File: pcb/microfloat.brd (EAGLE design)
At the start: 76.2 x 60.3 mm, 156 parts, among them J1 503182-1852, J2 1054291110, J3 USB4105_REVA, J4 1054291110, J5 JTAG-MINI, J6 1909763-1, J7 1054291110, J8 1054291110, T100 MMBT3906, U1 TXB0104PWR, U100 TPS54308DDCT, U101 LTC4419CMSEPBF, U102 MAX13237EETE, U103 TPS54308DDCT, U104 TPS54308DDCT, U105 TPS54308DDCT, U2 ICM-42688-P, U3 ATSAMD51N20A-AUT, U4 NEO-M8N-0, U5 BME280, Y1 ABS25-32.768KHZ-6-1-T

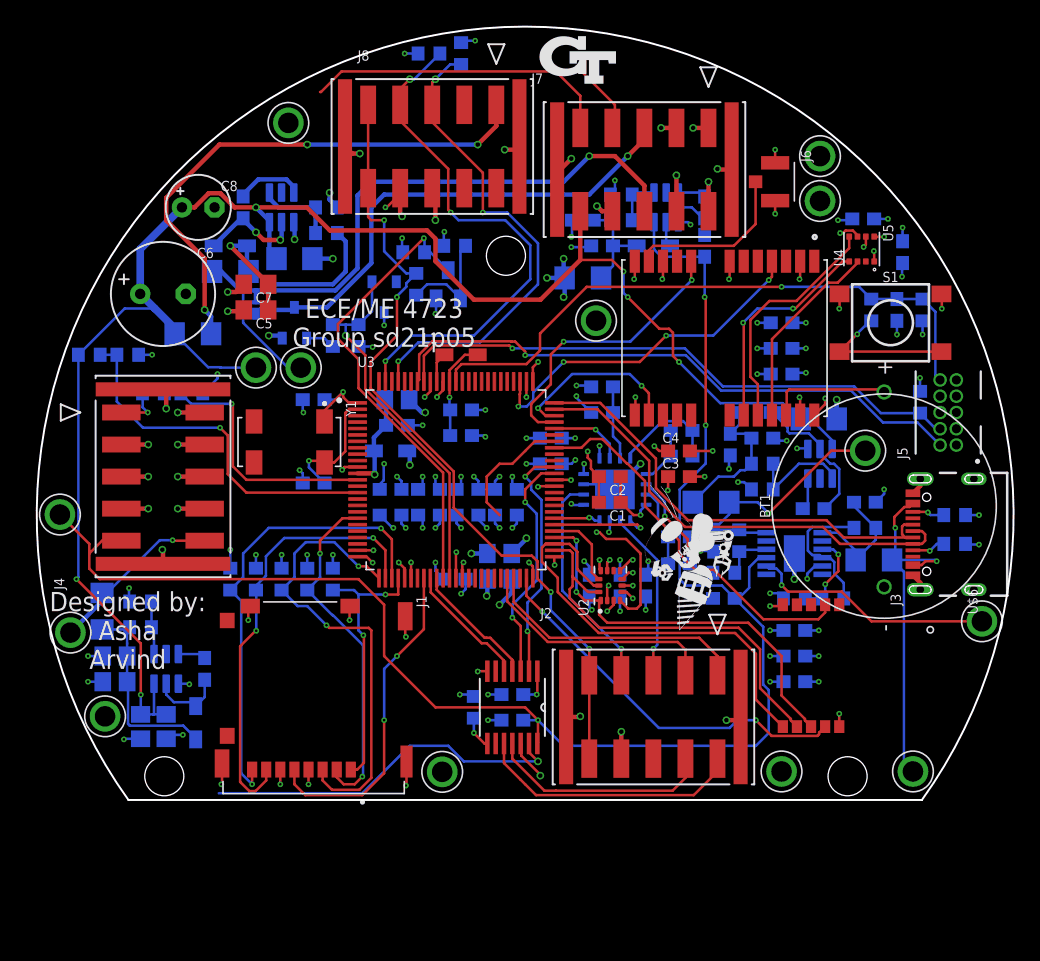
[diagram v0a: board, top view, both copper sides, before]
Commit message: More changes
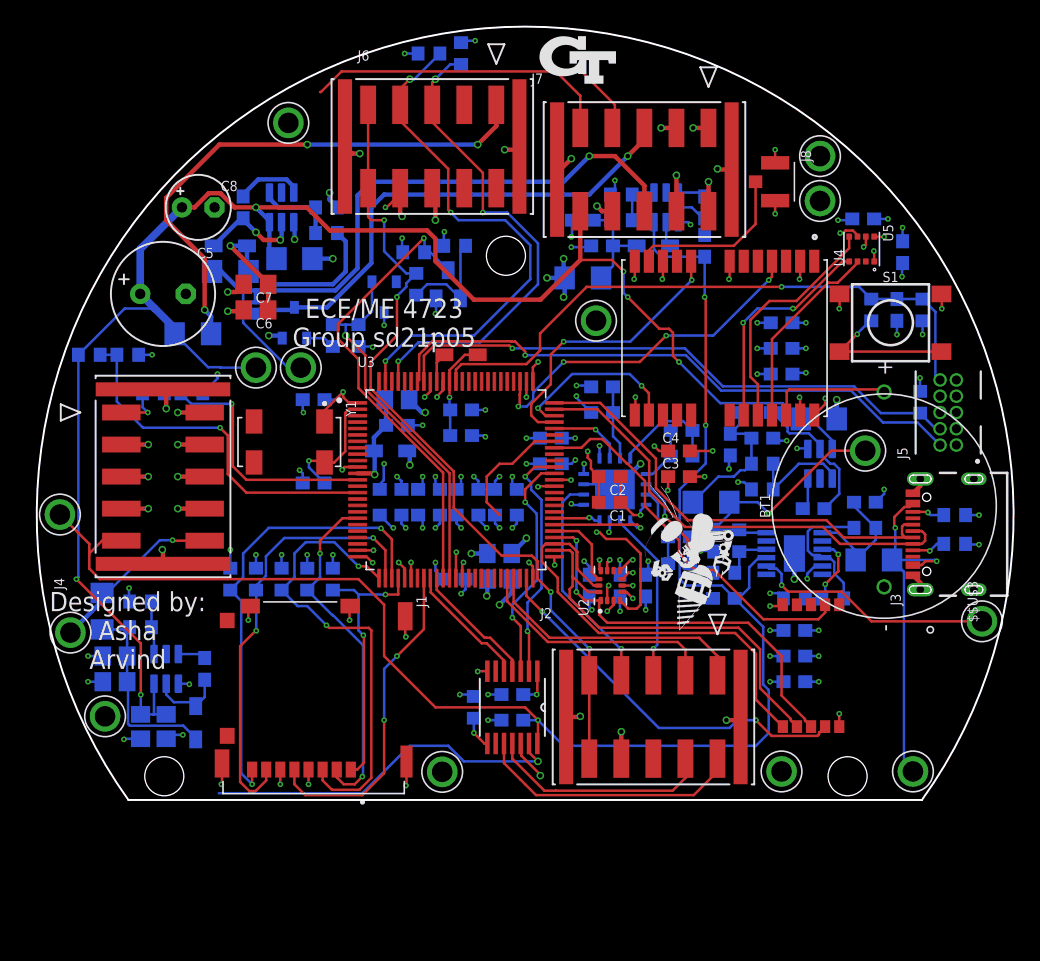
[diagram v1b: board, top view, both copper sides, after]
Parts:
- removed R103: 68k, rcl:R0603
- removed R104: 43k, rcl:R0603
- removed U$100: SQ2348ES-T1_GE3, microfloat:SOT-23-3
- removed U$101: GSOT04-E3-08, microfloat:SOT-23-3
- removed U$12, U$13: TEST_POINT, microfloat:TEST_POINT
- removed U$15: (no value), RoboJackets-Aesthetics:ROBOBUZZ_0.6X
- added $$$$U$3, $$$$U$4, $$$$U$5, $$U$1: TEST_POINT, microfloat:TEST_POINT
- added $$U$3: LR62E, microfloat:LR62E
- added R34: 1k', rcl:R0603
- added R35: 649, rcl:R0603
- $$U$10: value TEST_POINT -> SQ2348ES-T1_GE3; device microfloat:TEST_POINT -> microfloat:SOT-23-3
- $$U$11: value TEST_POINT -> GSOT04-E3-08; device microfloat:TEST_POINT -> microfloat:SOT-23-3
- C5: value 22uF -> 100uF; device rcl:C0805 -> rcl:E3,5-8
- C6: value 100uF -> 22uF; device rcl:E3,5-8 -> rcl:C0805
- J6: value 1909763-1 -> 1054291110; device microfloat:TE_1909763-1 -> microfloat:CON_1054291110_MOL
- J8: value 1054291110 -> 1909763-1; device microfloat:CON_1054291110_MOL -> microfloat:TE_1909763-1
- R1: value 649 -> 68k
- R2: value 1k' -> 43k
- U$6: value LR62E -> (none); device microfloat:LR62E -> RoboJackets-Aesthetics:ROBOBUZZ_0.6X
- moved $$U$4 66.6 mm to (-11.5, 20.8)
- moved R1 52.9 mm to (48.0, 23.5), turned to 180 degrees
- moved R2 49.8 mm to (45.0, 23.5), turned to 180 degrees
- moved $$U$10 45.6 mm to (6.00, 45.0), flipped to the bottom
- moved U$9 44.5 mm to (29.5, 45.2)
- moved U$8 27.4 mm to (6.50, 41.5)
- moved J6 22.6 mm to (21.8, 62.0), turned to 0 degrees
- moved J8 22.6 mm to (43.5, 56.0), turned to 270 degrees
- moved $$U$5 16.1 mm to (-12.3, 30.0)
- moved U$6 14.8 mm to (36.0, 21.0), turned to 0 degrees
- moved $$U$11 11.4 mm to (13.0, 47.0), flipped to the bottom, turned to 180 degrees
- moved C5 7.36 mm to (-4.25, 47.2), turned to 0 degrees
- moved C6 7.36 mm to (3.00, 46.0), turned to 180 degrees
- renumbered $$U$14 to $$U$7, $$U$16 to $$$$U$8, $$U$17 to $$$$U$6, $$U$18 to $$$$U$9, C100 to C16, C101 to C17, C102 to C13, C103 to C14, C104 to C9, C105 to C18, C106 to C15, C107 to C10, C108 to C19, C109 to C11, C110 to C12, C111 to C26, C112 to C27, C113 to C28, C114 to C32, C115 to C36, C116 to C24, C117 to C33, C118 to C22, C119 to C25, C120 to C30, C121 to C34, C122 to C37, C123 to C39, C124 to C21, C125 to C20, C126 to C31, C127 to C35, C128 to C38, C129 to C40, C130 to C41, C131 to C29, C132 to C23, C133 to C47, C134 to C46, C135 to C51, C136 to C52, C137 to C48, C138 to C54, C139 to C42, C140 to C49, C141 to C53, C142 to C55, C143 to C56, C144 to C50, C145 to C43, C146 to C44, C147 to C45, C148 to C58, C149 to C64, C150 to C57, C151 to C60, C152 to C62, C153 to C63, C154 to C59, C155 to C61, C156 to C65, CR100 to CR1, F100 to F1, F101 to F2, F102 to F3, F103 to F4, F104 to F5, F105 to F6, L100 to L2, L101 to L4, L102 to L3, L103 to L5, L104 to L6, R100 to R3, R101 to R4, R102 to R5, R105 to R13, R106 to R14, R107 to R15, R108 to R16, R109 to R17, R110 to R12, R111 to R6, R112 to R11, R113 to R8, R114 to R7, R115 to R9, R116 to R10, R117 to R18, R118 to R21, R119 to R22, R120 to R23, R121 to R24, R122 to R19, R123 to R20, R124 to R25, R125 to R26, R126 to R30, R127 to R31, R128 to R29, R129 to R32, R130 to R27, R131 to R33, R132 to R28, T100 to T1, U100 to U6, U101 to U8, U102 to U9, U103 to U7, U104 to U10, U105 to U11
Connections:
- net !SX-NRESET: now also $$U$3.P$2; no longer U$6.P$2
- net +12V: now also U$8.P$1; no longer U$12.P$1
- net +3V3: now also $$U$3.P$5, R34.2, R35.2; no longer R1.2, R2.2, U$6.P$5
- net +5V: now also $$U$5.P$1; no longer U$9.P$1
- net +6V: now also $$U$4.P$1; no longer U$8.P$1
- net ANT_SW: now also $$U$3.P$1; no longer U$6.P$1
- net CS_RAD: now also $$U$3.P$9; no longer U$6.P$9
- net GND: now also $$U$1.P$1, $$U$10.2, $$U$11.3, $$U$3.P$10, C5.-, C6.2, J6.11, J6.12, J6.8, J6.9, J8.2, J8.3, R2.1, U$9.P$1; no longer $$U$5.P$1, C5.2, C6.-, J6.2, J6.3, J8.11, J8.12, J8.8, J8.9, R104.1, U$100.2, U$101.3, U$13.P$1, U$6.P$10
- net GPS_ANT: now also J8.1; no longer J6.1
- net MISO_2: now also $$U$3.P$8; no longer U$6.P$8
- net MOSI_2: now also $$U$3.P$7; no longer U$6.P$7
- net N$17: now also C6.1; no longer C5.1
- net N$21: now also R1.2; no longer R103.2
- net N$22: now also R1.1, R2.2; no longer R103.1, R104.2
- net N$24: now also $$U$10.1; no longer U$100.1
- net PROBE: now also J6.10, J6.5; no longer J8.10, J8.5
- net RAD_BUSY: now also $$U$3.P$3; no longer U$6.P$3
- net RREF+: now also J6.3, R34.1; no longer J8.3, R2.1
- net RSENSE+: now also J6.4, R35.1; no longer J8.4, R1.1
- net SCLK_2: now also $$U$3.P$6; no longer U$6.P$6
- net SOLENOID: now also $$U$11.1; no longer U$101.1
- net SOL_TRIG: now also $$U$10.3; no longer U$100.3
- net VBATT: now also $$$$U$5.P$1, C5.+; no longer $$U$11.P$1, C6.+
- net VBATT_5V: now also $$$$U$4.P$1; no longer $$U$10.P$1
- net VBUS: now also $$$$U$3.P$1; no longer $$U$4.P$1
- net VIN: now also J6.1; no longer J8.1

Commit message: no airwires, clearance issues, dimensions, wire stubs
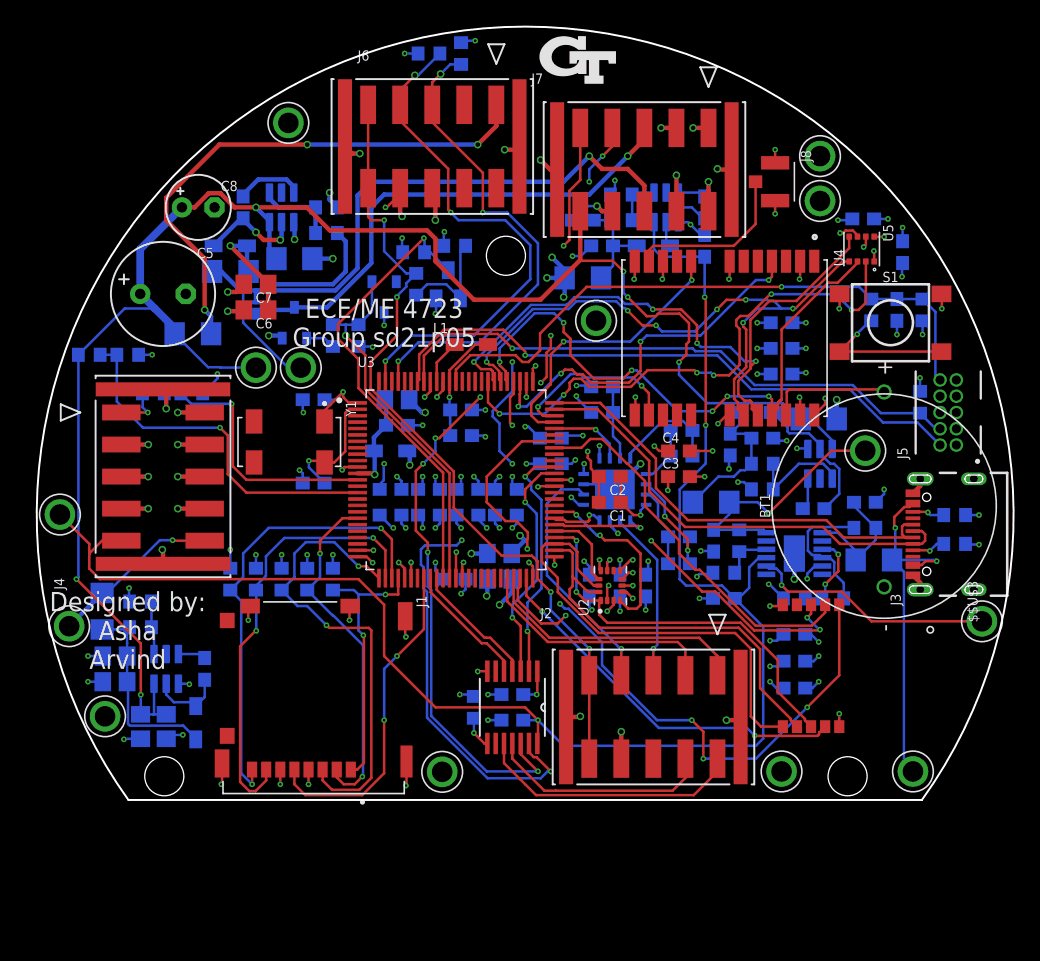
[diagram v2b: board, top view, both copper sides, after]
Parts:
- removed U$6: (no value), RoboJackets-Aesthetics:ROBOBUZZ_0.6X
- moved L1 1.13 mm to (19.8, 43.3)
- moved $$U$4 0.51 mm to (-11.6, 21.3)
- moved C9 0.50 mm to (45.0, 16.5)
- moved C10 0.40 mm to (45.0, 18.6)
- moved C11 0.30 mm to (45.0, 20.7)
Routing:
- net UART_RX_M_B: track 9.27 -> 68.3 mm, vias 1 -> 9
- net ANT_SW: track 9.82 -> 57.0 mm, vias 0 -> 5
- net CS_PHT: track 0.00 -> 42.8 mm, vias 0 -> 6
- net RAD_BUSY: track 0.00 -> 37.2 mm, vias 0 -> 4
- net MOSI_1: track 15.2 -> 47.1 mm, vias 0 -> 6
- net MISO_1: track 18.6 -> 49.8 mm, vias 0 -> 4
- net CS_GPS: track 0.00 -> 31.2 mm, vias 0 -> 2
- net SCLK_1: track 17.5 -> 47.9 mm, vias 2 -> 7
- net UART_TX_M_B: track 52.9 -> 69.9 mm, vias 1 -> 5
- net IMU_INT: track 10.1 -> 14.1 mm, vias 1 -> 2
- net GND: track 187.9 -> 190.8 mm, vias 132 -> 131
- net VBATT: track 135.8 -> 138.3 mm
- net +3V3: track 74.9 -> 77.0 mm
- net T_OUT: track 17.4 -> 19.3 mm
- net TX_READY: track 27.5 -> 29.4 mm
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
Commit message: BEEG Capacitor
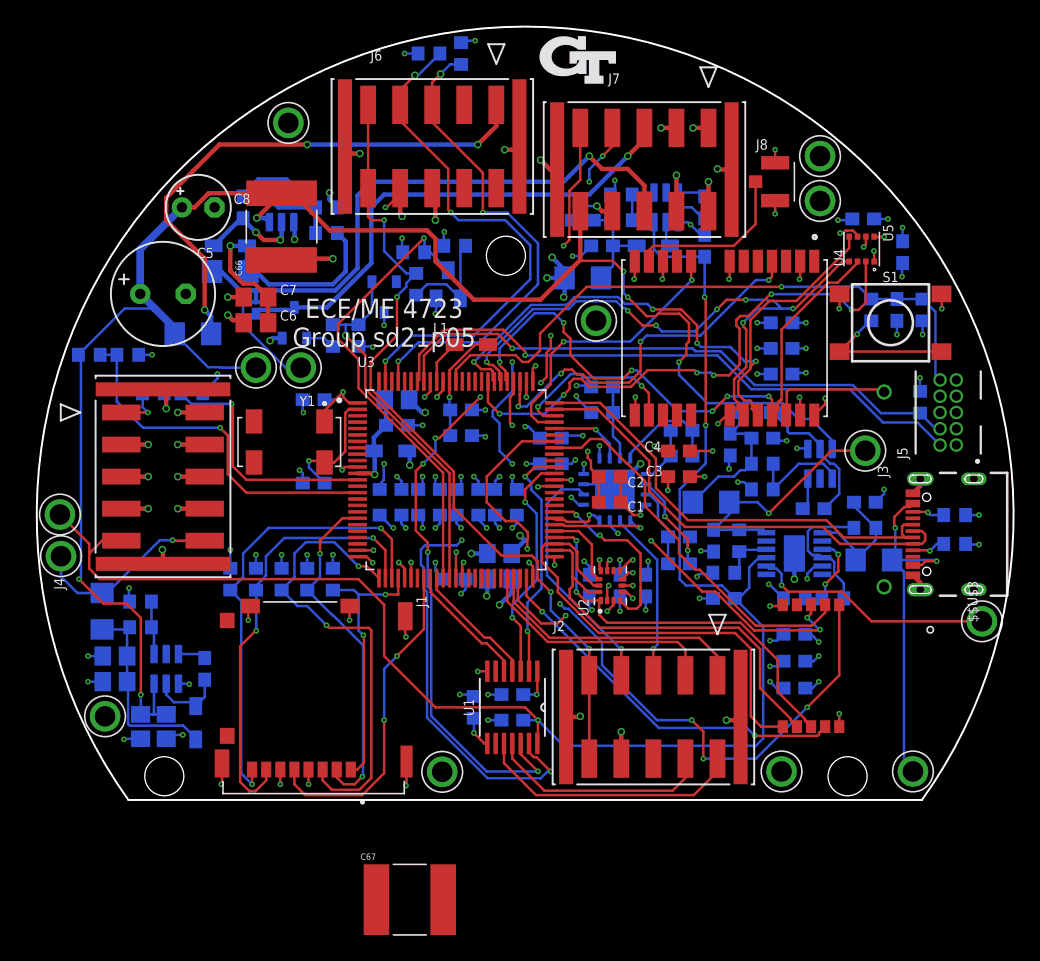
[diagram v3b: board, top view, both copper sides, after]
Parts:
- removed C42, C64: 33uF, rcl:C1206
- added C66, C67: KCM55TR7YA336MH01L, microfloat:CAPC6153X500N
- moved $$U$4 5.50 mm to (-12.2, 26.8)
- moved C6 1.00 mm to (3.00, 45.0)
- moved C7 1.00 mm to (3.00, 47.0)
- flipped BT1 to the bottom
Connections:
- net GND: now also C66.1, C67.1; no longer C42.2, C64.2
- net VBATT: now also C66.2, C67.2; no longer C42.1, C64.1
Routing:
- net +6V: track 13.4 -> 15.0 mm
- net N$17: track 21.2 -> 22.8 mm
- net GND: track 190.8 -> 191.6 mm, vias 131 -> 130
- net VBATT: track 138.3 -> 138.8 mm
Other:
- board text removed: "Designed by: Asha Arvind"
